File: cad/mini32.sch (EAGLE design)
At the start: 51 parts, among them CN1 MICROSDPLAIN, J1 HEADER-5X1, Q1 MOSFETSOT-23, SW2 SWITCHKMR211, SW3 SWITCHKMR211, U1 STM32F411/48, U2 MPU-9150, U3 ADP5062, U4 MCP1824, X1 12MHz, X2 32k768

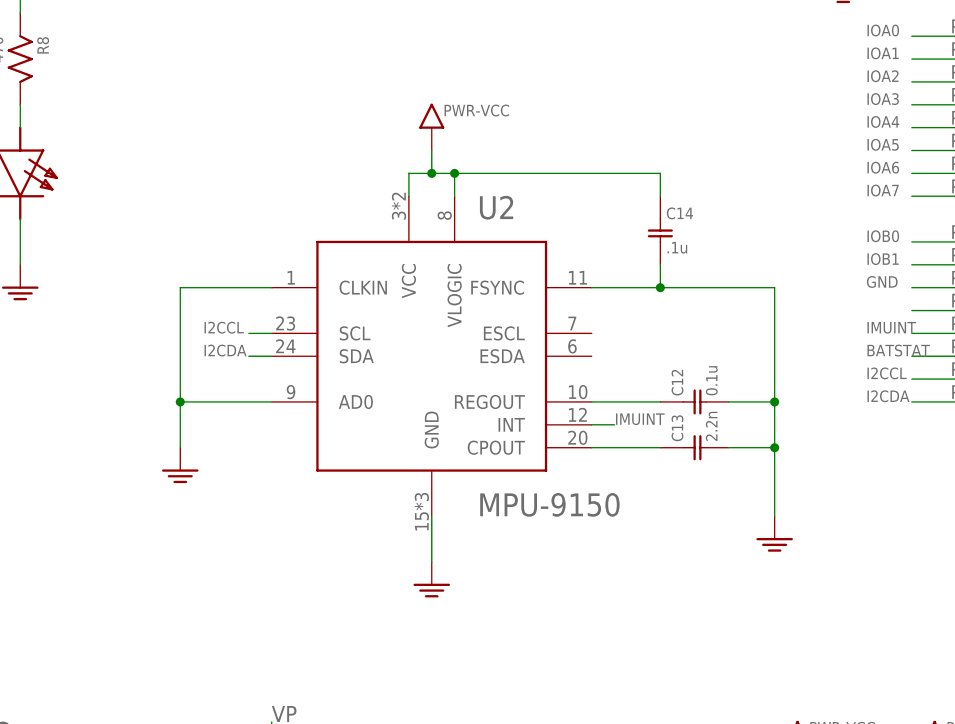
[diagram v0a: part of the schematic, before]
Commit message: lsm303d
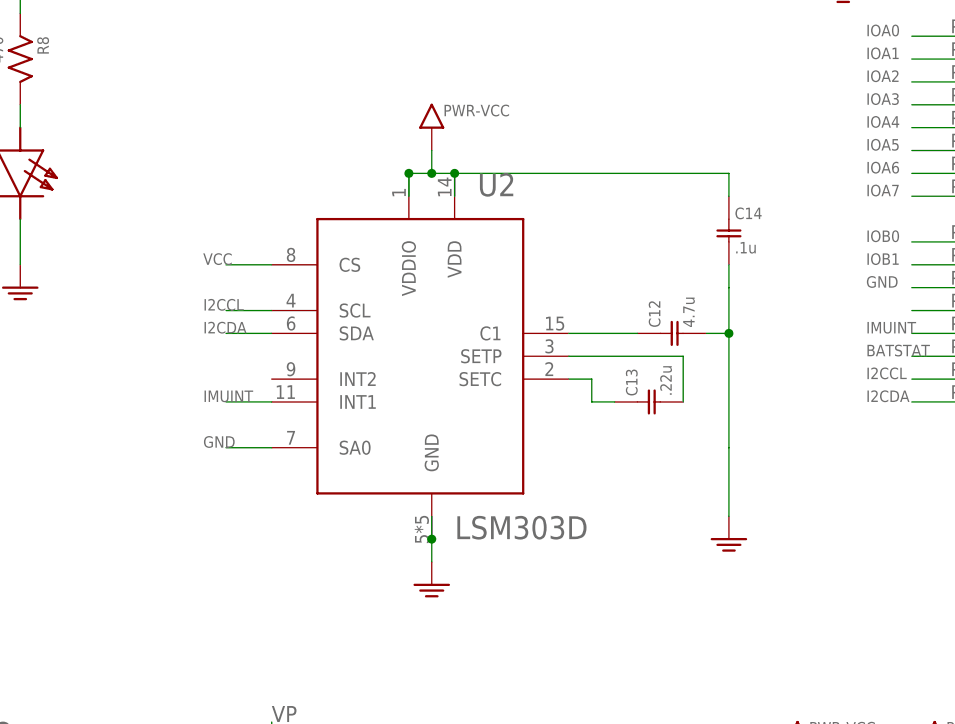
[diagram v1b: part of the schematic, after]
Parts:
- C12: value 0.1u -> 4.7u
- C13: value 2.2n -> .22u
- U2: value MPU-9150 -> LSM303D; device jaw:MPU-9150 -> jaw:LSM303D
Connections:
- new net N$1: C12.P$1, U2.C1
- net GND: now also U2.SA0; no longer C13.P$2, U2.AD0, U2.CLKIN, U2.FSYNC
- net IMUINT: now also U2.INT1; no longer U2.INT
- net N$2: now also C13.P$2, U2.SETP; no longer C12.P$1, U2.REGOUT
- net N$4: now also U2.SETC; no longer U2.CPOUT
- net VCC: now also U2.CS, U2.VDD, U2.VDDIO; no longer U2.VCC, U2.VLOGIC
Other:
- moved on the sheet: C12, C13, C14
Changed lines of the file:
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@@
 <part name="U$2" library="adafruit" deviceset="FIDUCIAL" device=""/>
 <part name="U$3" library="adafruit" deviceset="FIDUCIAL" device=""/>
-<part name="U2" library="jaw" deviceset="MPU-9150" device=""/>
-<part name="C12" library="jaw" deviceset="C" device="0603" value="0.1u"/>
-<part name="C13" library="jaw" deviceset="C" device="0603" value="2.2n"/>
+<part name="C12" library="jaw" deviceset="C" device="0603" value="4.7u"/>
+<part name="C13" library="jaw" deviceset="C" device="0603" value=".22u"/>
 <part name="C14" library="jaw" deviceset="C" device="0603" value=".1u"/>
 <part name="GND12" library="jaw" deviceset="PWR-GND" device=""/>
 <part name="GND14" library="jaw" deviceset="PWR-GND" device=""/>
-<part name="GND15" library="jaw" deviceset="PWR-GND" device=""/>
 <part name="VCC4" library="jaw" deviceset="PWR-VCC" device=""/>
 <part name="GND19" library="jaw" deviceset="PWR-GND" device=""/>
@@
 <part name="B1" library="jaw" deviceset="BATTERY" device="-CR2016"/>
 <part name="X1" library="jaw" deviceset="RESONATOR" device="CTCE" value="12MHz"/>
+<part name="U2" library="jaw" deviceset="LSM303D" device=""/>
 </parts>
 <sheets>
@@
 <instance part="U$2" gate="G$1" x="269.24" y="40.64"/>
 <instance part="U$3" gate="G$1" x="261.62" y="40.64"/>
-<instance part="U2" gate="G$1" x="99.06" y="106.68"/>
-<instance part="C12" gate="G$1" x="129.54" y="101.6" rot="R90"/>
-<instance part="C13" gate="G$1" x="129.54" y="96.52" rot="R90"/>
-<instance part="C14" gate="G$1" x="124.46" y="119.38"/>
+<instance part="C12" gate="G$1" x="127" y="109.22" rot="R90"/>
+<instance part="C13" gate="G$1" x="124.46" y="101.6" rot="R90"/>
+<instance part="C14" gate="G$1" x="132.08" y="119.38"/>
 <instance part="GND12" gate="G$1" x="99.06" y="81.28"/>
-<instance part="GND14" gate="G$1" x="137.16" y="86.36"/>
-<instance part="GND15" gate="G$1" x="71.12" y="93.98"/>
+<instance part="GND14" gate="G$1" x="132.08" y="86.36"/>
 <instance part="VCC4" gate="G$1" x="99.06" y="132.08"/>
 <instance part="GND19" gate="G$1" x="30.48" y="167.64"/>
@@
 <instance part="B1" gate="G$1" x="226.06" y="170.18"/>
 <instance part="X1" gate="G$1" x="144.78" y="160.02"/>
+<instance part="U2" gate="G$1" x="99.06" y="106.68"/>
 </instances>
 <busses>
@@
 </segment>
 <segment>
+<pinref part="GND12" gate="G$1" pin="GND"/>
+<wire x1="99.06" y1="88.9" x2="99.06" y2="86.36" width="0.1524" layer="91"/>
 <pinref part="U2" gate="G$1" pin="GND"/>
-<pinref part="GND12" gate="G$1" pin="GND"/>
-<wire x1="99.06" y1="88.9" x2="99.06" y2="83.82" width="0.1524" layer="91"/>
+<wire x1="99.06" y1="86.36" x2="99.06" y2="83.82" width="0.1524" layer="91"/>
+<junction x="99.06" y="86.36"/>
 </segment>
 <segment>
 <pinref part="C12" gate="G$1" pin="P$2"/>
-<wire x1="132.08" y1="101.6" x2="137.16" y2="101.6" width="0.1524" layer="91"/>
-<wire x1="137.16" y1="101.6" x2="137.16" y2="96.52" width="0.1524" layer="91"/>
-<pinref part="C13" gate="G$1" pin="P$2"/>
-<wire x1="137.16" y1="96.52" x2="132.08" y2="96.52" width="0.1524" layer="91"/>
+<wire x1="129.54" y1="109.22" x2="132.08" y2="109.22" width="0.1524" layer="91"/>
+<wire x1="132.08" y1="109.22" x2="132.08" y2="96.52" width="0.1524" layer="91"/>
 <pinref part="GND14" gate="G$1" pin="GND"/>
-<wire x1="137.16" y1="96.52" x2="137.16" y2="88.9" width="0.1524" layer="91"/>
-<junction x="137.16" y="96.52"/>
-<pinref part="U2" gate="G$1" pin="FSYNC"/>
-<wire x1="116.84" y1="114.3" x2="124.46" y2="114.3" width="0.1524" layer="91"/>
-<wire x1="124.46" y1="114.3" x2="137.16" y2="114.3" width="0.1524" layer="91"/>
-<wire x1="137.16" y1="114.3" x2="137.16" y2="101.6" width="0.1524" layer="91"/>
-<junction x="137.16" y="101.6"/>
+<wire x1="132.08" y1="96.52" x2="132.08" y2="88.9" width="0.1524" layer="91"/>
+<wire x1="132.08" y1="114.3" x2="132.08" y2="109.22" width="0.1524" layer="91"/>
+<junction x="132.08" y="109.22"/>
 <pinref part="C14" gate="G$1" pin="P$2"/>
-<wire x1="124.46" y1="116.84" x2="124.46" y2="114.3" width="0.1524" layer="91"/>
-<junction x="124.46" y="114.3"/>
-</segment>
-<segment>
-<pinref part="U2" gate="G$1" pin="AD0"/>
-<pinref part="GND15" gate="G$1" pin="GND"/>
-<wire x1="81.28" y1="101.6" x2="71.12" y2="101.6" width="0.1524" layer="91"/>
-<wire x1="71.12" y1="101.6" x2="71.12" y2="96.52" width="0.1524" layer="91"/>
-<pinref part="U2" gate="G$1" pin="CLKIN"/>
-<wire x1="81.28" y1="114.3" x2="71.12" y2="114.3" width="0.1524" layer="91"/>
-<wire x1="71.12" y1="114.3" x2="71.12" y2="101.6" width="0.1524" layer="91"/>
-<junction x="71.12" y="101.6"/>
+<wire x1="132.08" y1="116.84" x2="132.08" y2="114.3" width="0.1524" layer="91"/>
 </segment>
 <segment>
@@
 <wire x1="17.78" y1="38.1" x2="15.24" y2="38.1" width="0.1524" layer="91"/>
 <label x="12.7" y="38.1" size="1.27" layer="95"/>
+</segment>
+<segment>
+<pinref part="U2" gate="G$1" pin="SA0"/>
+<wire x1="81.28" y1="96.52" x2="76.2" y2="96.52" width="0.1524" layer="91"/>
+<label x="73.66" y="96.52" size="1.27" layer="95"/>
 </segment>
 </net>
@@
 <segment>
 <pinref part="C14" gate="G$1" pin="P$1"/>
-<wire x1="124.46" y1="124.46" x2="124.46" y2="127" width="0.1524" layer="91"/>
-<pinref part="U2" gate="G$1" pin="VLOGIC"/>
-<wire x1="124.46" y1="127" x2="101.6" y2="127" width="0.1524" layer="91"/>
+<wire x1="132.08" y1="124.46" x2="132.08" y2="127" width="0.1524" layer="91"/>
+<wire x1="132.08" y1="127" x2="101.6" y2="127" width="0.1524" layer="91"/>
 <wire x1="101.6" y1="127" x2="101.6" y2="124.46" width="0.1524" layer="91"/>
-<pinref part="U2" gate="G$1" pin="VCC"/>
 <wire x1="101.6" y1="127" x2="99.06" y2="127" width="0.1524" layer="91"/>
 <wire x1="99.06" y1="127" x2="96.52" y2="127" width="0.1524" layer="91"/>
@@
 <wire x1="99.06" y1="129.54" x2="99.06" y2="127" width="0.1524" layer="91"/>
 <junction x="99.06" y="127"/>
+<pinref part="U2" gate="G$1" pin="VDDIO"/>
+<junction x="96.52" y="127"/>
+<pinref part="U2" gate="G$1" pin="VDD"/>
 </segment>
 <segment>
@@
 <label x="246.38" y="177.8" size="1.27" layer="95"/>
 <pinref part="J1" gate="G$1" pin="1"/>
+</segment>
+<segment>
+<pinref part="U2" gate="G$1" pin="CS"/>
+<wire x1="81.28" y1="116.84" x2="76.2" y2="116.84" width="0.1524" layer="91"/>
+<label x="73.66" y="116.84" size="1.27" layer="95"/>
 </segment>
 </net>
@@
 </segment>
 </net>
-<net name="N$2" class="0">
-<segment>
-<pinref part="U2" gate="G$1" pin="REGOUT"/>
-<pinref part="C12" gate="G$1" pin="P$1"/>
-<wire x1="116.84" y1="101.6" x2="124.46" y2="101.6" width="0.1524" layer="91"/>
-</segment>
-</net>
-<net name="N$4" class="0">
-<segment>
-<pinref part="U2" gate="G$1" pin="CPOUT"/>
-<pinref part="C13" gate="G$1" pin="P$1"/>
-<wire x1="116.84" y1="96.52" x2="124.46" y2="96.52" width="0.1524" layer="91"/>
-</segment>
-</net>
 <net name="I2CCL" class="0">
-<segment>
-<pinref part="U2" gate="G$1" pin="SCL"/>
-<wire x1="81.28" y1="109.22" x2="78.74" y2="109.22" width="0.1524" layer="91"/>
-<label x="73.66" y="109.22" size="1.27" layer="95"/>
-</segment>
 <segment>
 <pinref part="U1" gate="G$1" pin="PB6"/>
@@
 <label x="10.16" y="48.26" size="1.27" layer="95"/>
 </segment>
+<segment>
+<pinref part="U2" gate="G$1" pin="SCL"/>
+<wire x1="81.28" y1="111.76" x2="76.2" y2="111.76" width="0.1524" layer="91"/>
+<label x="73.66" y="111.76" size="1.27" layer="95"/>
+</segment>
 </net>
 <net name="I2CDA" class="0">
-<segment>
-<pinref part="U2" gate="G$1" pin="SDA"/>
-<wire x1="81.28" y1="106.68" x2="78.74" y2="106.68" width="0.1524" layer="91"/>
-<label x="73.66" y="106.68" size="1.27" layer="95"/>
-</segment>
 <segment>
 <pinref part="U1" gate="G$1" pin="PB7"/>
@@
 <label x="10.16" y="45.72" size="1.27" layer="95"/>
 </segment>
+<segment>
+<pinref part="U2" gate="G$1" pin="SDA"/>
+<wire x1="81.28" y1="109.22" x2="76.2" y2="109.22" width="0.1524" layer="91"/>
+<label x="73.66" y="109.22" size="1.27" layer="95"/>
+</segment>
 </net>
 <net name="DPYDC" class="0">
@@
 </segment>
 <segment>
-<pinref part="U2" gate="G$1" pin="INT"/>
-<wire x1="116.84" y1="99.06" x2="119.38" y2="99.06" width="0.1524" layer="91"/>
-<label x="119.38" y="99.06" size="1.27" layer="95"/>
+<pinref part="U2" gate="G$1" pin="INT1"/>
+<wire x1="81.28" y1="101.6" x2="76.2" y2="101.6" width="0.1524" layer="91"/>
+<label x="73.66" y="101.6" size="1.27" layer="95"/>
 </segment>
 </net>
@@
 </segment>
 </net>
+<net name="N$1" class="0">
+<segment>
+<pinref part="C12" gate="G$1" pin="P$1"/>
+<pinref part="U2" gate="G$1" pin="C1"/>
+<wire x1="121.92" y1="109.22" x2="114.3" y2="109.22" width="0.1524" layer="91"/>
+</segment>
+</net>
+<net name="N$2" class="0">
+<segment>
+<pinref part="U2" gate="G$1" pin="SETP"/>
+<wire x1="114.3" y1="106.68" x2="127" y2="106.68" width="0.1524" layer="91"/>
+<pinref part="C13" gate="G$1" pin="P$2"/>
+<wire x1="127" y1="106.68" x2="127" y2="101.6" width="0.1524" layer="91"/>
+</segment>
+</net>
+<net name="N$4" class="0">
+<segment>
+<pinref part="C13" gate="G$1" pin="P$1"/>
+<wire x1="119.38" y1="101.6" x2="116.84" y2="101.6" width="0.1524" layer="91"/>
+<wire x1="116.84" y1="101.6" x2="116.84" y2="104.14" width="0.1524" layer="91"/>
+<pinref part="U2" gate="G$1" pin="SETC"/>
+<wire x1="116.84" y1="104.14" x2="114.3" y2="104.14" width="0.1524" layer="91"/>
+</segment>
+</net>
